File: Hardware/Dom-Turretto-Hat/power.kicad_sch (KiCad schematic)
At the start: 26 parts, among them J3 Barrel_Jack_Switch, J4 Conn_01x02, U3 LM22679TJ-5.0{slash}NOPB, U4 LTC4451AV#TRMPBF, U5 LTC4451AV#TRMPBF, U6 LT1963AxST-3.3, U7 LTC4411ES5TRMPBF

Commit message: Updated schematic
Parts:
- J4: footprint (none) -> Connector_AMASS:AMASS_XT60-M_1x02_P7.20mm_Vertical
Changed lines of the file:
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@@
       (effects (font (size 1.27 1.27)) (justify left))
     )
-    (property "Footprint" "" (id 2) (at 58.42 54.61 0)
+    (property "Footprint" "Connector_AMASS:AMASS_XT60-M_1x02_P7.20mm_Vertical" (id 2) (at 58.42 54.61 0)
       (effects (font (size 1.27 1.27)) hide)
     )

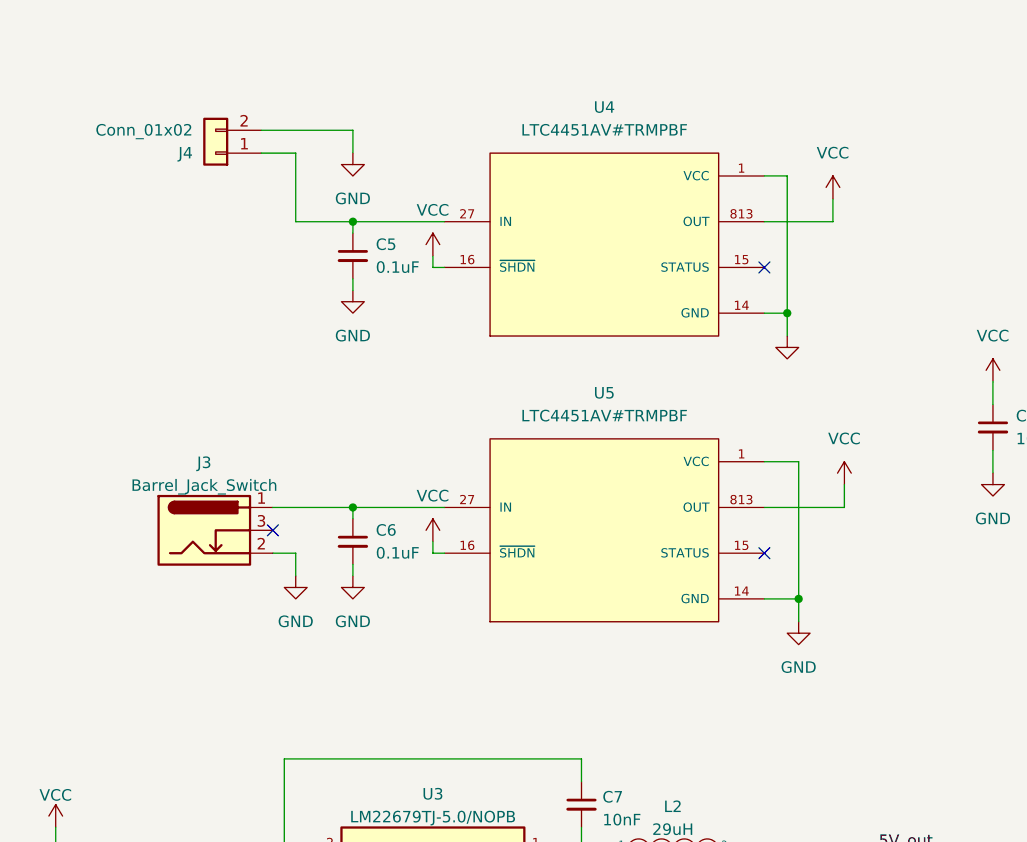
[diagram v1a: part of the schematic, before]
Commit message: Update components
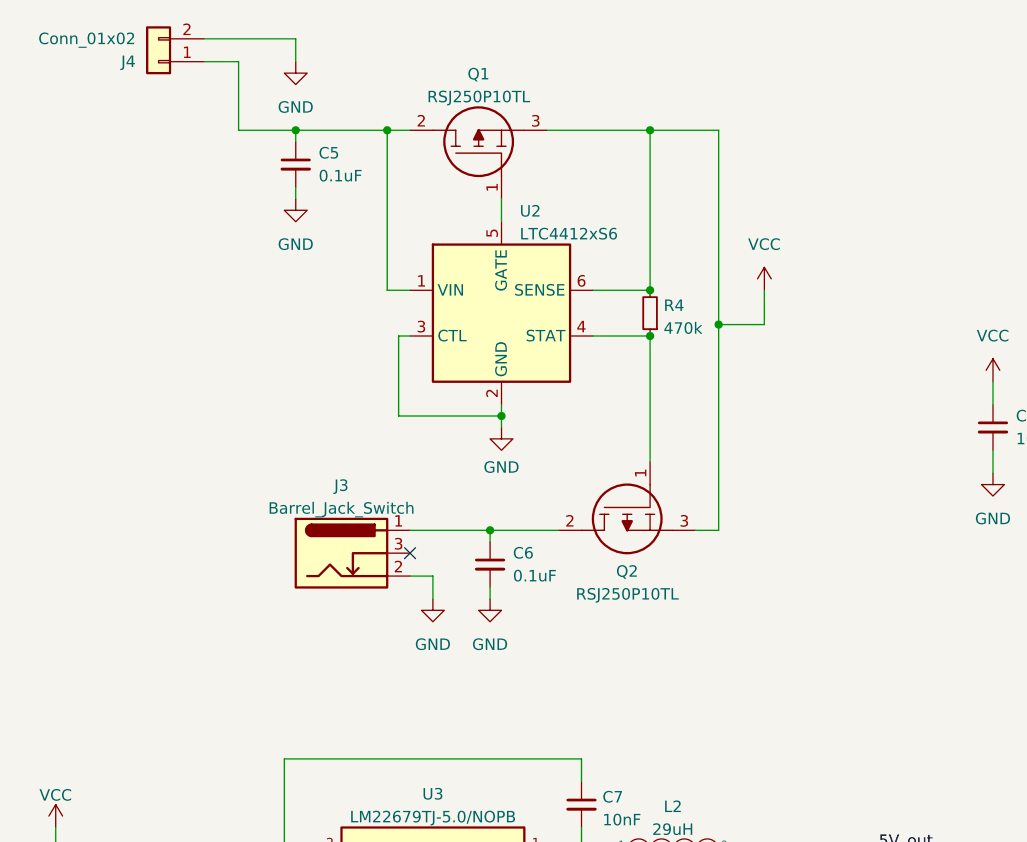
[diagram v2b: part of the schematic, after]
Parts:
- removed U4, U5: LTC4451AV#TRMPBF, iclr:IC_LTC4451AV#TRMPBF, symbol iclr:LTC4451AV#TRMPBF
- added Q1, Q2: RSJ250P10TL, Package_TO_SOT_SMD:TO-263-3_TabPin2, symbol iclr:RSJ250P10TL
- added R4: 470k, Resistor_SMD:R_0603_1608Metric, symbol Device:R_Small
- added U2: LTC4412xS6, Package_TO_SOT_SMD:TSOT-23-6, symbol Power_Management:LTC4412xS6
- J4: footprint Connector_AMASS:AMASS_XT60-M_1x02_P7.20mm_Vertical -> Connector_AMASS:AMASS_XT60-F_1x02_P7.20mm_Vertical
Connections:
- net GND: now also U2.2 (GND), U2.3 (CTL)
- net VCC: now also Q1.3, Q2.3, R4.2, U2.6 (SENSE)
- net at C6.1, J3.1: now also Q2.2
- net at C5.1, J4.1 (Pin_1): now also Q1.2, U2.1 (VIN)
- new net: Q2.1, R4.1, U2.4 (STAT)
- new net: Q1.1, U2.5 (GATE)
- no-connect marks 6 -> 4
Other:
- moved on the sheet: C5, C6, J3, J4
